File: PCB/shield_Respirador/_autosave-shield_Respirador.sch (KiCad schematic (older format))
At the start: 34 parts, among them P1 Digital, P10 CONN_01X01, P11 CONN_01X01, P12 CONN_01X01, P13 CONN_01X01, P2 Power, P3 Analog, P4 Analog, P5 PWM, P6 PWM, P7 Communication, P8 CONN_01X01, P9 CONN_01X01

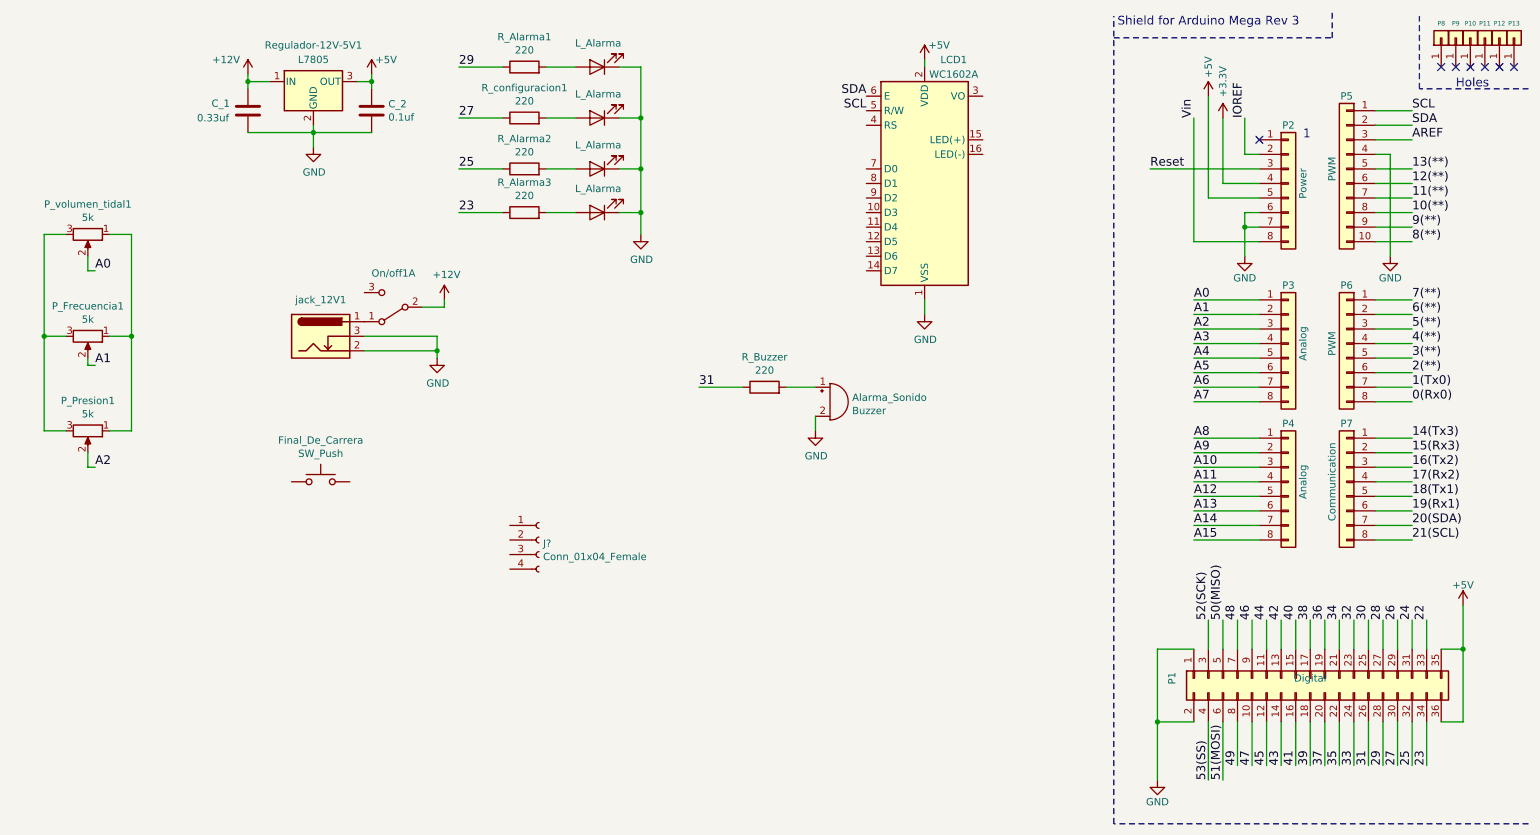
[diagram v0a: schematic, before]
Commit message: version 0.4
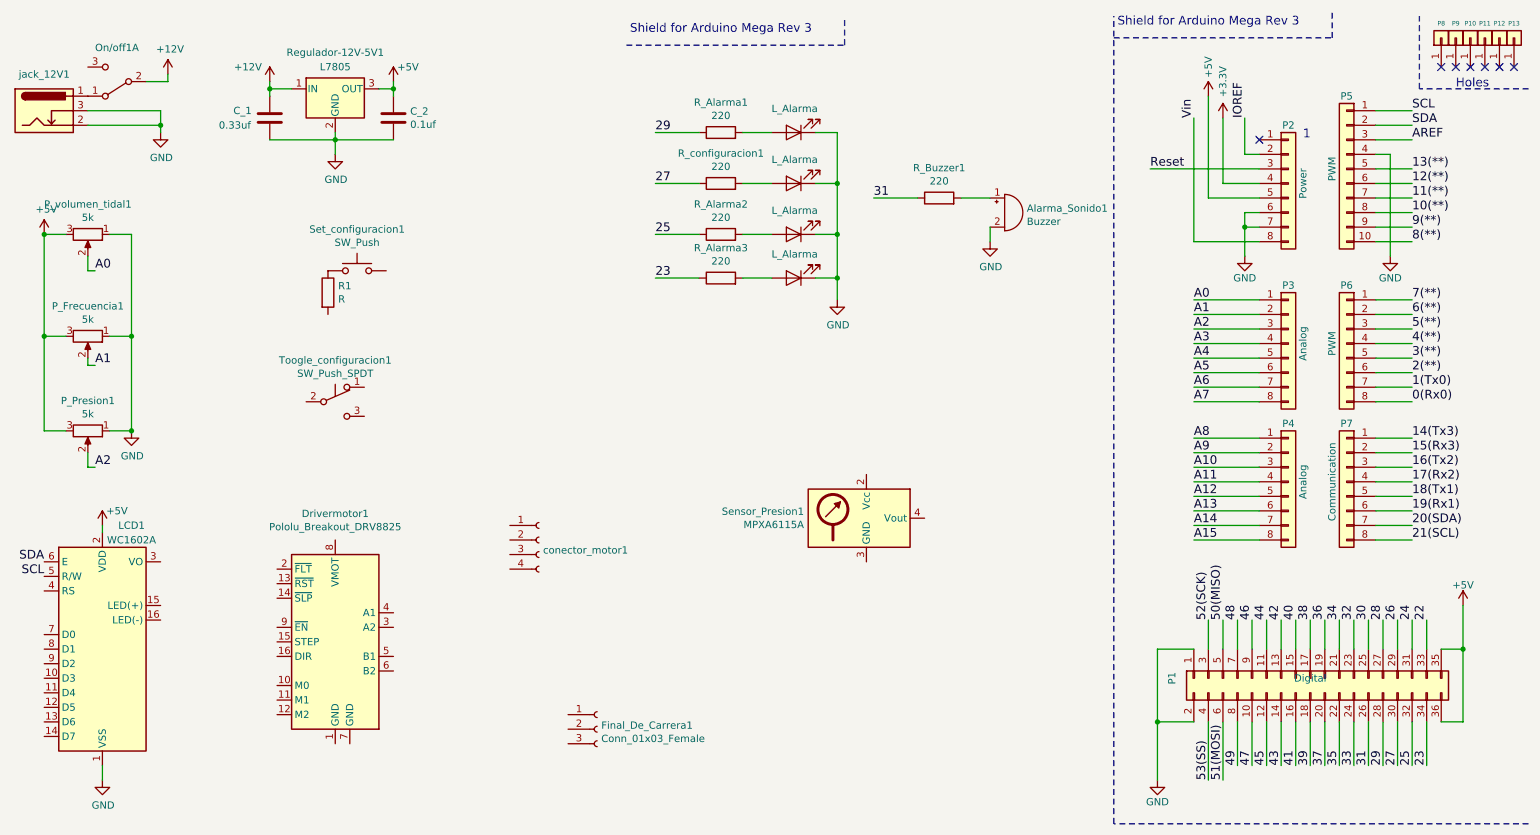
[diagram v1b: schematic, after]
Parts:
- removed Final_De_Carrera: SW_Push, symbol Switch:SW_Push
- added Drivermotor1: Pololu_Breakout_DRV8825, Module:Pololu_Breakout-16_15.2x20.3mm, symbol Driver_Motor:Pololu_Breakout_DRV8825
- added Final_De_Carrera1: Conn_01x03_Female, Connector_PinSocket_2.00mm:PinSocket_1x03_P2.00mm_Vertical, symbol Connector:Conn_01x03_Female
- added R1: R, symbol Device:R
- added Sensor_Presion1: MPXA6115A, Package_DIP:DIP-8_W7.62mm_LongPads, symbol Sensor_Pressure:MPXA6115A
- added Set_configuracion1: SW_Push, TerminalBlock:TerminalBlock_bornier-2_P5.08mm, symbol Switch:SW_Push
- added Toogle_configuracion1: SW_Push_SPDT, TerminalBlock:TerminalBlock_bornier-3_P5.08mm, symbol Switch:SW_Push_SPDT
- Alarma_Sonido1: renamed from Alarma_Sonido; footprint (none) -> Buzzer_Beeper:MagneticBuzzer_ProSignal_ABI-009-RC
- On/off1: footprint Connector:Banana_Jack_3Pin -> TerminalBlock:TerminalBlock_bornier-3_P5.08mm
- conector_motor1: renamed from J?; footprint (none) -> Connector_PinSocket_2.00mm:PinSocket_1x04_P2.00mm_Vertical
- renumbered R_Buzzer to R_Buzzer1
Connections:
- net +5V: now also P_Frecuencia1.3, P_Presion1.3, P_volumen_tidal1.3
- net GND: now also P_Frecuencia1.1, P_Presion1.1, P_volumen_tidal1.1
- new net: R1.1, Set_configuracion1.1
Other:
- moved on the sheet: Alarma_Sonido1, C_1, C_2, LCD1, On/off1A, R_Alarma1, R_Alarma2, R_Alarma3, R_Buzzer1, R_configuracion1, Regulador-12V-5V1, jack_12V1
